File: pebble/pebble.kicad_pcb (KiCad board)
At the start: 4 copper layers, 129 x 129 mm, 160 parts, among them J1 UART, J2 GPS, J3 USB_C_Receptacle_USB2.0_16P, J4 BAT, J5 Conn_01x03_Pin, Q1 BSS84, Q2 BSS123, U1 TPS61023DRLR, U2 TPS563200, U3 ESP32-C6-MINI-1, U4 BMI270, U5 MAX-M8Q, U6 BMM350, U7 MAX77751CEFG+, U8 LPV521, U9 MAX4906ELB+T

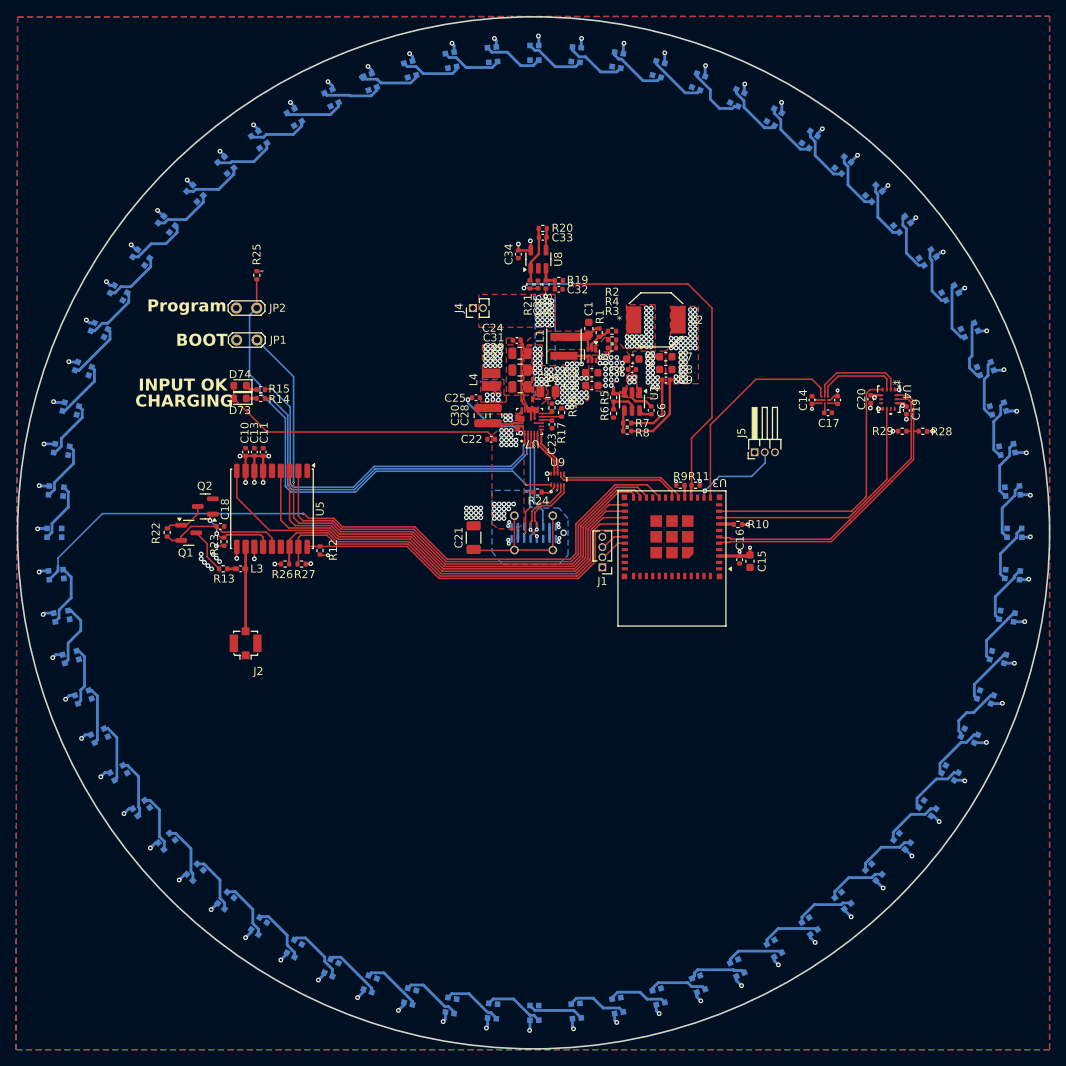
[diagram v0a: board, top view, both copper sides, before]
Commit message: finalize rev0
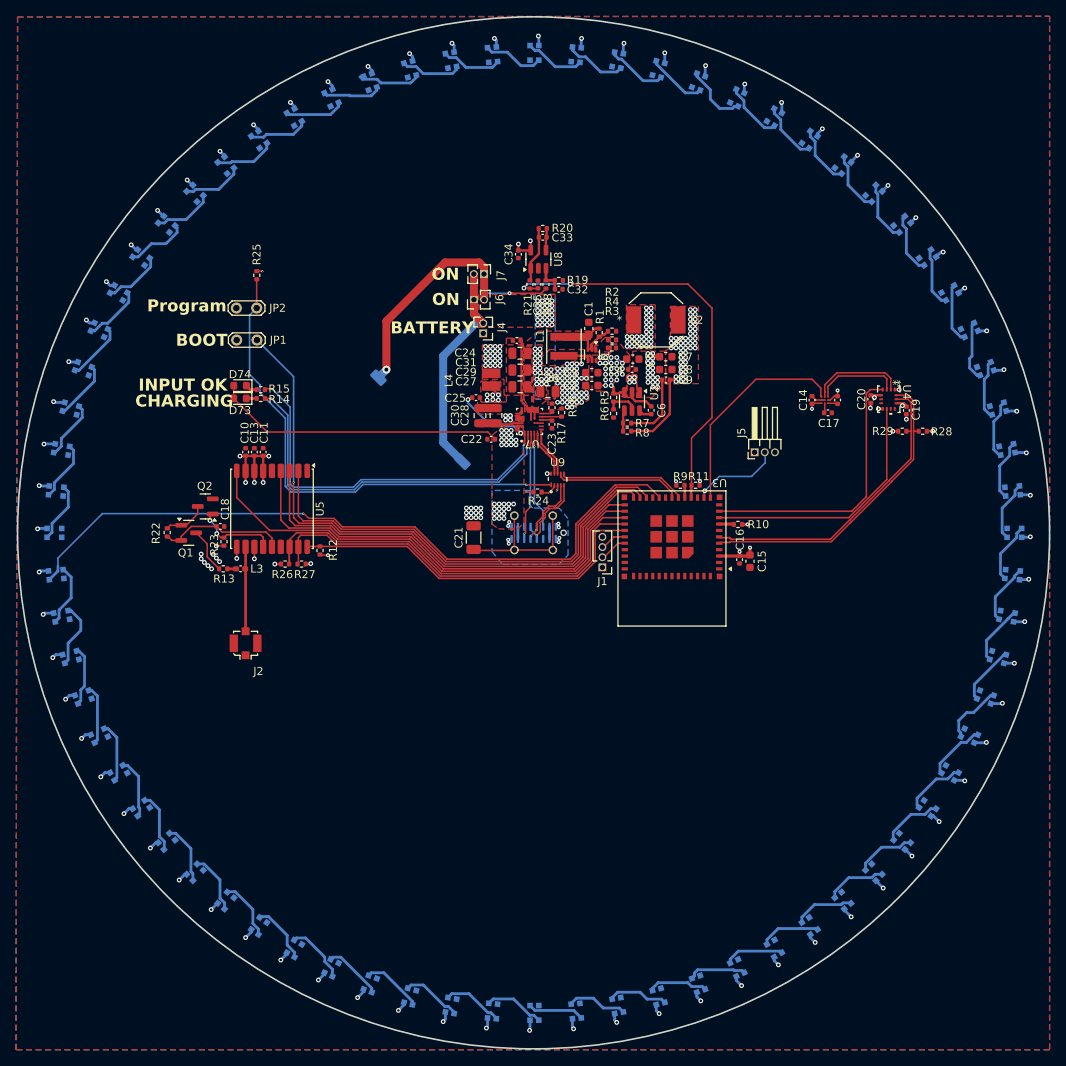
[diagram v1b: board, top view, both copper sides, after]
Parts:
- added J6: ON, Connector_PinHeader_1.27mm:PinHeader_1x02_P1.27mm_Vertical, F.Cu at (142.5, 70.8)
- added J7: ON, Connector_PinHeader_1.27mm:PinHeader_1x02_P1.27mm_Vertical, F.Cu at (143.8, 67.7)
- added SW1: SW_Reed, kicad-symbols:59170-1-S-00-D, B.Cu at (135.9, 85.9)
- moved J4 3.42 mm to (143.7, 75.1), turned to 180 degrees
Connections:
- C26 pad 1: Net-(J4-Pin_2) -> Net-(J6-Pin_2)
- J3 pad A6: /charger/DN_in -> /charger/DP_in
- J3 pad A7: /charger/DP_in -> /charger/DN_in
- J3 pad B6: /charger/DN_in -> /charger/DP_in
- J3 pad B7: /charger/DP_in -> /charger/DN_in
- R18 pad 2: Net-(J4-Pin_2) -> Net-(J6-Pin_2)
- U7 pad 13: Net-(J4-Pin_2) -> Net-(J6-Pin_2)
- U7 pad 14: Net-(J4-Pin_2) -> Net-(J6-Pin_2)
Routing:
- net Net-(J6-Pin_2): track 0.00 -> 36.2 mm, vias 0 -> 37
- net Net-(J4-Pin_2): track 1.56 -> 30.3 mm, vias 36 -> 0
- net Net-(JP2-B): track 63.6 -> 62.2 mm
- added copper zone on B.Cu, net Net-(J6-Pin_2)
- added copper zone on F.Cu, net Net-(J6-Pin_2)
- removed copper zone on B.Cu, net Net-(J4-Pin_2)
- removed copper zone on F.Cu, net Net-(J4-Pin_2)
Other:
- board text added: "BATTERY"
- board text added: "ON"
- board text added: "Pebble rev0 designed by @Yatekii"
